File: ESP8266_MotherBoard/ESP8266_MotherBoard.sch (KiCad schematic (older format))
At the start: 67 parts, among them CN1 DIP-BLACK-FEMALE-HEADER-VERT_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, IC1 ADXL345, J1 Screw_Terminal_01x03, J10 Screw_Terminal_01x06, J11 Screw_Terminal_01x12, J2 DIP-BLACK-MALE-HEADER-VERT_4P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, J3 Screw_Terminal_01x02, J5 DIP-BLACK-MALE-HEADER-R_A_3P-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, J6 Screw_Terminal_01x02, J7 DIP-BLACK-MALE-HEADER-R_A_3P-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, J8 DIP-BLACK-FEMALE-HEADER-VERT_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, J9 Screw_Terminal_01x12, Q1 MMBT2907, Q10 MMBT2222, Q2 MMBT2907, Q3 MMBT2907, Q4 MMBT2907, Q5 Q_PMOS_GDS, Q6 MMBT2222, Q9 Q_PMOS_GDS, U1 LM75B, U2 NodeMCU1.0(ESP-12E), U3 L9110, U4 XL6009_Module, U5 L78L33_SOT89

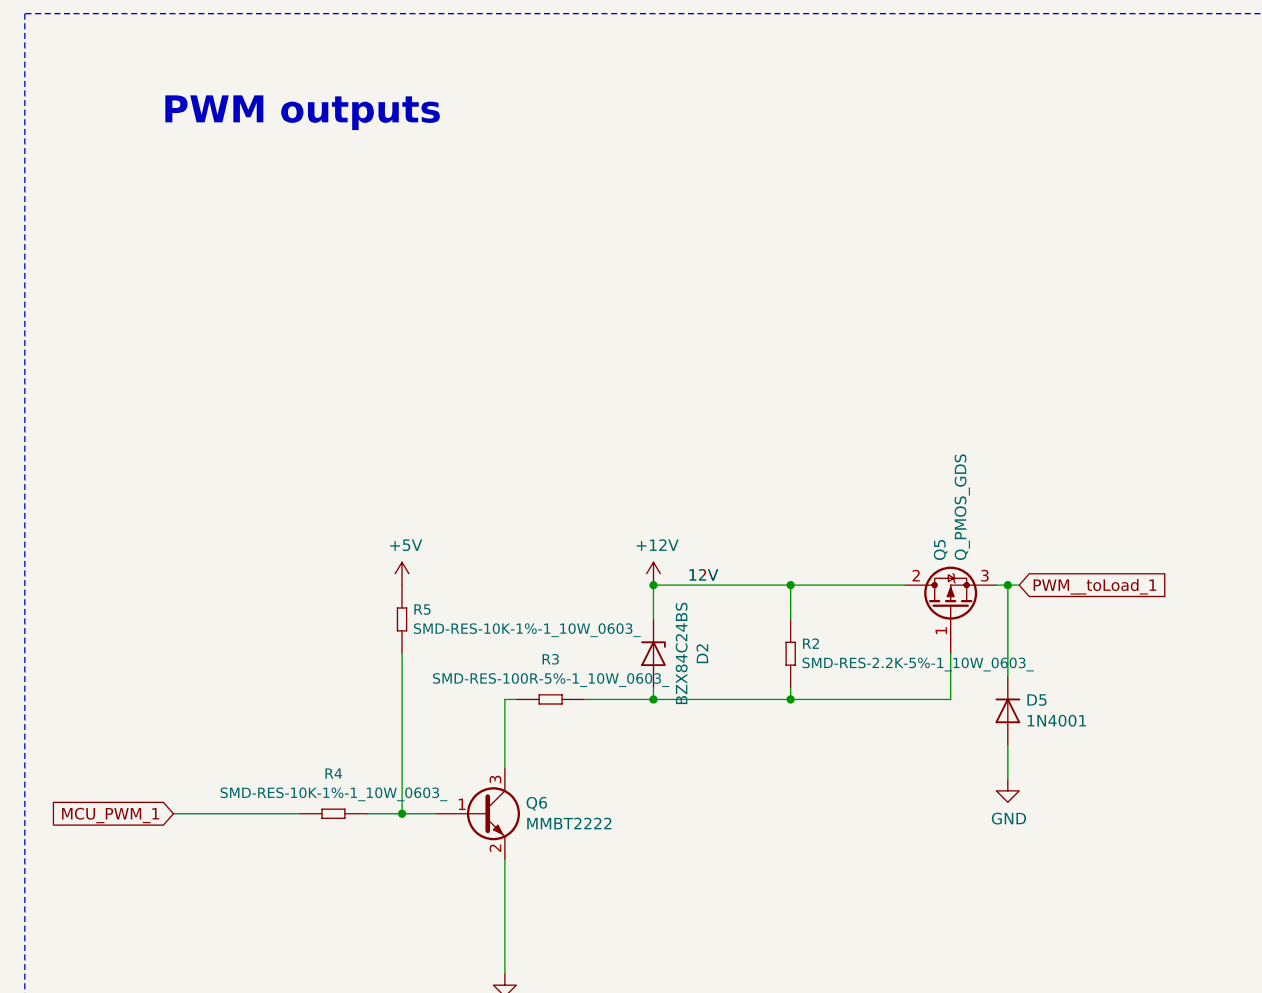
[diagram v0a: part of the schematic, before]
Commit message: test branch sch and board changed
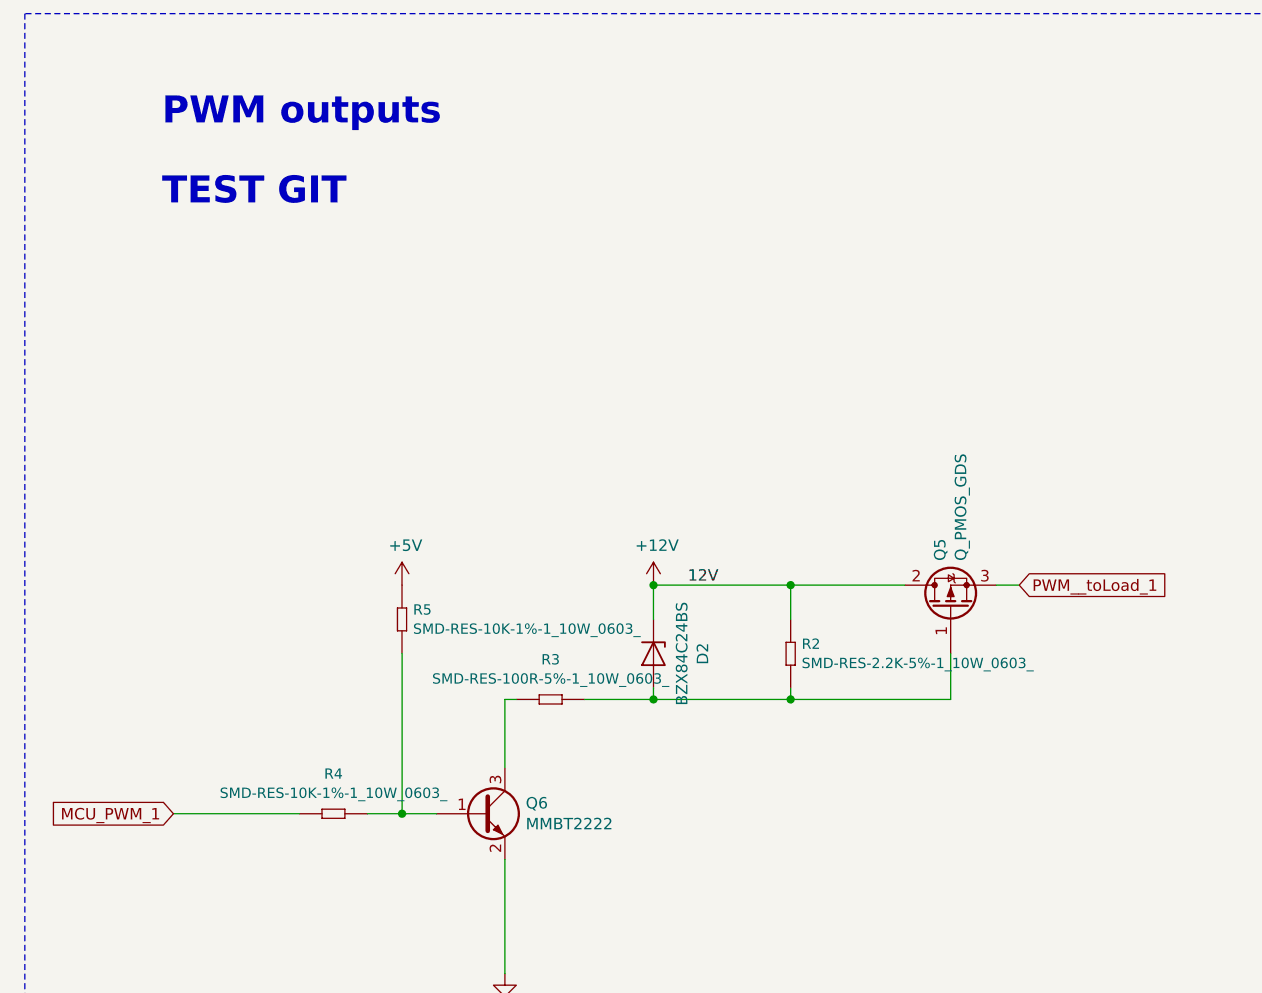
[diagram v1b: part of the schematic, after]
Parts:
- removed D5: 1N4001, OPL_Discrete_Semiconductor:DO-41, symbol Diode:1N4001
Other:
- note added: "TEST GIT"
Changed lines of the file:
@@
 Wire Wire Line
 	18550 7300 19250 7300
-Wire Wire Line
-	19550 6800 19500 6800
 Text GLabel 15850 7800 0    50   Input ~ 0
 MCU_PWM_1
@@
 Wire Wire Line
 	25400 6850 25350 6850
-$Comp
-L Diode:1N4001 D5
-U 1 1 5DBBA1F3
-P 19500 7350
-F 0 "D5" V 19454 7429 50  0000 L CNN
-F 1 "1N4001" V 19545 7429 50  0000 L CNN
-F 2 "OPL_Discrete_Semiconductor:DO-41" H 19500 7175 50  0001 C CNN
-F 3 "http://www.vishay.com/docs/88503/1n4001.pdf" H 19500 7350 50  0001 C CNN
-	1    19500 7350
-	0    1    1    0
-$EndComp
-$Comp
-L power:GND #PWR0111
-U 1 1 5DBBA1FA
-P 19500 7650
-F 0 "#PWR0111" H 19500 7400 50  0001 C CNN
-F 1 "GND" H 19505 7477 50  0000 C CNN
-F 2 "" H 19500 7650 50  0001 C CNN
-F 3 "" H 19500 7650 50  0001 C CNN
-	1    19500 7650
-	1    0    0    -1
-$EndComp
-Wire Wire Line
-	19500 7500 19500 7650
-Wire Wire Line
-	19500 7200 19500 6800
-Connection ~ 19500 6800
-Wire Wire Line
-	19500 6800 19450 6800
 Text Label 18100 6800 0    50   ~ 0
 12V
@@
 	16850 7800 17000 7800
 $Comp
-L power:+5V #PWR?
+L power:+5V #PWR0155
 U 1 1 61115E76
 P 16850 6800
-F 0 "#PWR?" H 16850 6650 50  0001 C CNN
+F 0 "#PWR0155" H 16850 6650 50  0001 C CNN
 F 1 "+5V" H 16865 6973 50  0000 C CNN
 F 2 "" H 16850 6800 50  0001 C CNN
@@
 	22750 7150 22750 7850
 $Comp
-L power:+5V #PWR?
+L power:+5V #PWR0156
 U 1 1 61123AA3
 P 22750 6850
-F 0 "#PWR?" H 22750 6700 50  0001 C CNN
+F 0 "#PWR0156" H 22750 6700 50  0001 C CNN
 F 1 "+5V" H 22765 7023 50  0000 C CNN
 F 2 "" H 22750 6850 50  0001 C CNN
@@
 	1    0    0    -1
 $EndComp
+Text Notes 15800 5150 0    118  ~ 24
+TEST GIT
+Wire Wire Line
+	19450 6800 19550 6800
 $EndSCHEMATC

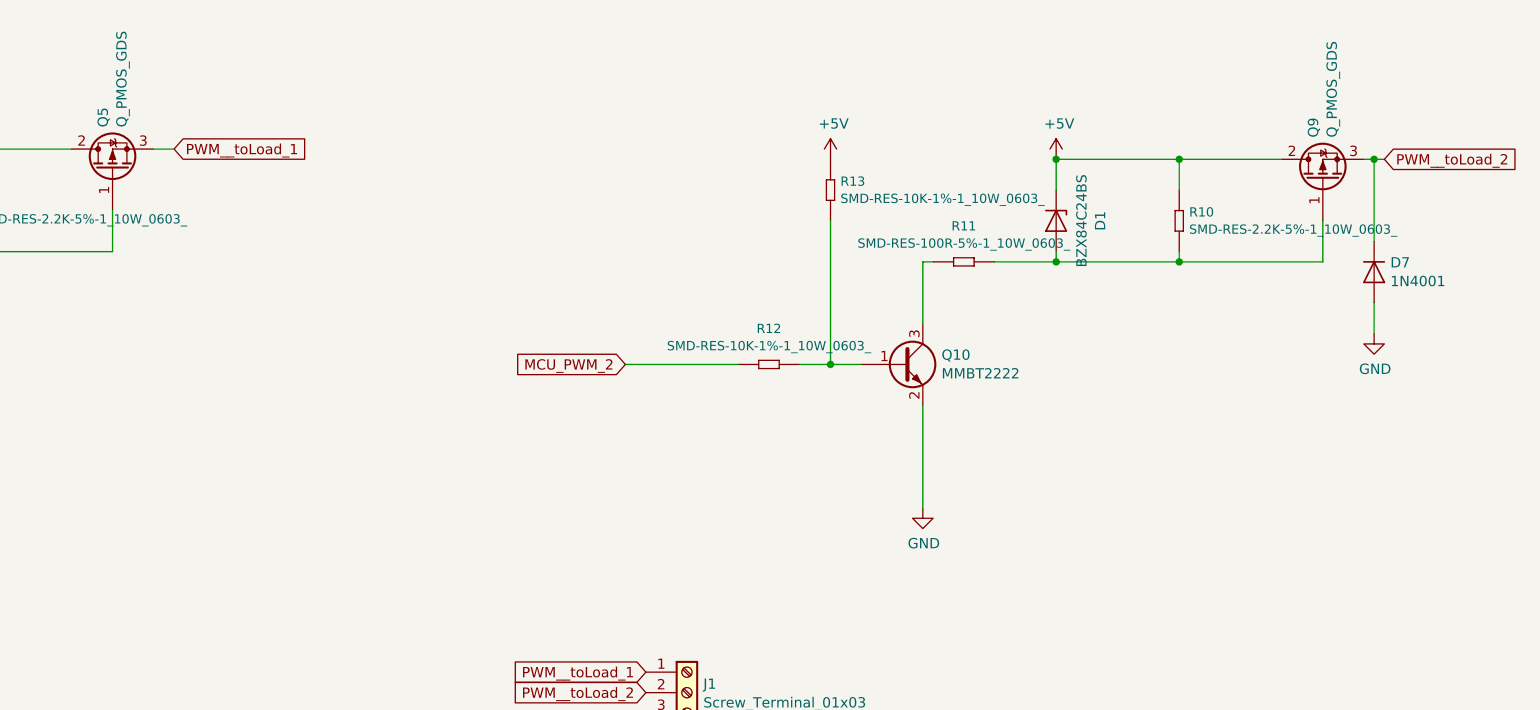
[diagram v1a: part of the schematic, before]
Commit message: added D3 ro PWM modul
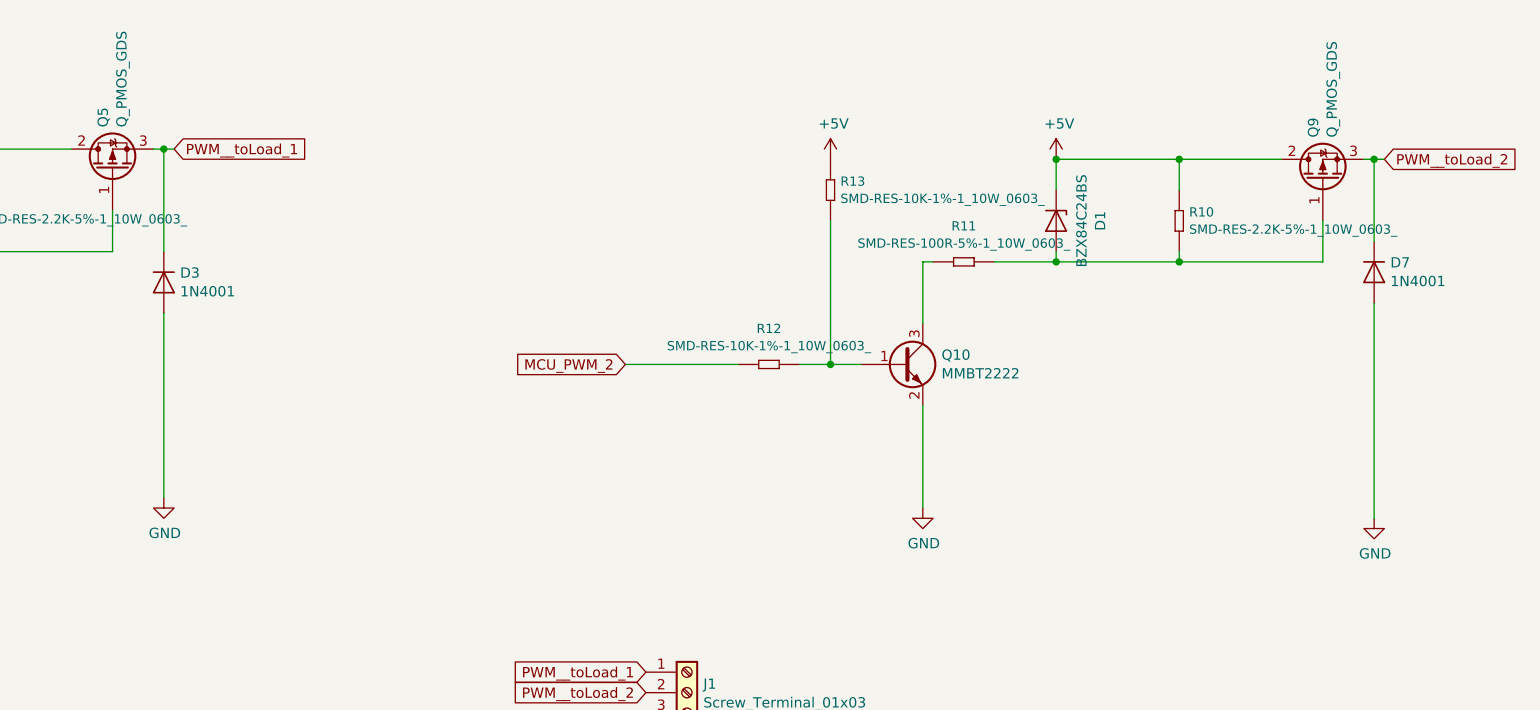
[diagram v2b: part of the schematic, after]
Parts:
- added D3: 1N4001, OPL_Discrete_Semiconductor:DO-41, symbol Diode:1N4001
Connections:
- net GND: now also D3.2 (A)
- net PWM__toLoad_1: now also D3.1 (K)
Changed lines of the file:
@@
-$EndComp
-$Comp
-L Device:Q_PMOS_GDS Q9
-U 1 1 5DB806F6
-P 25150 6950
-F 0 "Q9" H 25356 6996 50  0000 L CNN
-F 1 "Q_PMOS_GDS" H 25356 6905 50  0000 L CNN
-F 2 "Package_TO_SOT_SMD:TO-252-3_TabPin4" H 25350 7050 50  0001 C CNN
-F 3 "~" H 25150 6950 50  0001 C CNN
-	1    25150 6950
-	0    -1   -1   0
 $EndComp
 $Comp
@@
 Wire Wire Line
 	24450 7350 25150 7350
-Wire Wire Line
-	25450 6850 25400 6850
 Text GLabel 21750 7850 0    50   Input ~ 0
 MCU_PWM_2
@@
 	0    1    1    0
 $EndComp
-$Comp
-L power:GND #PWR0109
-U 1 1 5DBAF1B1
-P 25400 7700
-F 0 "#PWR0109" H 25400 7450 50  0001 C CNN
-F 1 "GND" H 25405 7527 50  0000 C CNN
-F 2 "" H 25400 7700 50  0001 C CNN
-F 3 "" H 25400 7700 50  0001 C CNN
-	1    25400 7700
-	1    0    0    -1
-$EndComp
-Wire Wire Line
-	25400 7550 25400 7700
-Wire Wire Line
-	25400 7250 25400 6850
-Connection ~ 25400 6850
-Wire Wire Line
-	25400 6850 25350 6850
 Text Label 18100 6800 0    50   ~ 0
 12V
@@
 Text GLabel 11750 19500 0    50   Input ~ 0
 Analog_input
-Text GLabel 25450 6850 2    50   Input ~ 0
-PWM__toLoad_2
 $Comp
 L Connector:Screw_Terminal_01x03 J1
@@
 TEST GIT
 Wire Wire Line
-	19450 6800 19550 6800
+	19450 6800 19500 6800
+$Comp
+L power:GND #PWR0109
+U 1 1 5DBAF1B1
+P 25400 8600
+F 0 "#PWR0109" H 25400 8350 50  0001 C CNN
+F 1 "GND" H 25405 8427 50  0000 C CNN
+F 2 "" H 25400 8600 50  0001 C CNN
+F 3 "" H 25400 8600 50  0001 C CNN
+	1    25400 8600
+	1    0    0    -1
+$EndComp
+Wire Wire Line
+	25400 7550 25400 8600
+Wire Wire Line
+	25450 6850 25400 6850
+Wire Wire Line
+	25400 7250 25400 6850
+Connection ~ 25400 6850
+Wire Wire Line
+	25400 6850 25350 6850
+Text GLabel 25450 6850 2    50   Input ~ 0
+PWM__toLoad_2
+$Comp
+L Device:Q_PMOS_GDS Q9
+U 1 1 5DB806F6
+P 25150 6950
+F 0 "Q9" H 25356 6996 50  0000 L CNN
+F 1 "Q_PMOS_GDS" H 25356 6905 50  0000 L CNN
+F 2 "Package_TO_SOT_SMD:TO-252-3_TabPin4" H 25350 7050 50  0001 C CNN
+F 3 "~" H 25150 6950 50  0001 C CNN
+	1    25150 6950
+	0    -1   -1   0
+$EndComp
+$Comp
+L Diode:1N4001 D3
+U 1 1 61104467
+P 19500 7450
+F 0 "D3" V 19454 7529 50  0000 L CNN
+F 1 "1N4001" V 19545 7529 50  0000 L CNN
+F 2 "OPL_Discrete_Semiconductor:DO-41" H 19500 7275 50  0001 C CNN
+F 3 "http://www.vishay.com/docs/88503/1n4001.pdf" H 19500 7450 50  0001 C CNN
+	1    19500 7450
+	0    1    1    0
+$EndComp
+Wire Wire Line
+	19500 6800 19500 7300
+Connection ~ 19500 6800
+Wire Wire Line
+	19500 6800 19550 6800
+$Comp
+L power:GND #PWR0111
+U 1 1 61110983
+P 19500 8500
+F 0 "#PWR0111" H 19500 8250 50  0001 C CNN
+F 1 "GND" H 19505 8327 50  0000 C CNN
+F 2 "" H 19500 8500 50  0001 C CNN
+F 3 "" H 19500 8500 50  0001 C CNN
+	1    19500 8500
+	1    0    0    -1
+$EndComp
+Wire Wire Line
+	19500 7600 19500 8500
 $EndSCHEMATC
